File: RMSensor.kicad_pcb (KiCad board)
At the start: 2 copper layers, 32 x 32 mm, 26 parts, among them J1 Conn_01x02, J2 Conn_01x02, J3 Conn_01x04, U1 OPA209AID, U2 OPA2350UA, U3 MC78L05_SO8, U4 TLE2425xD

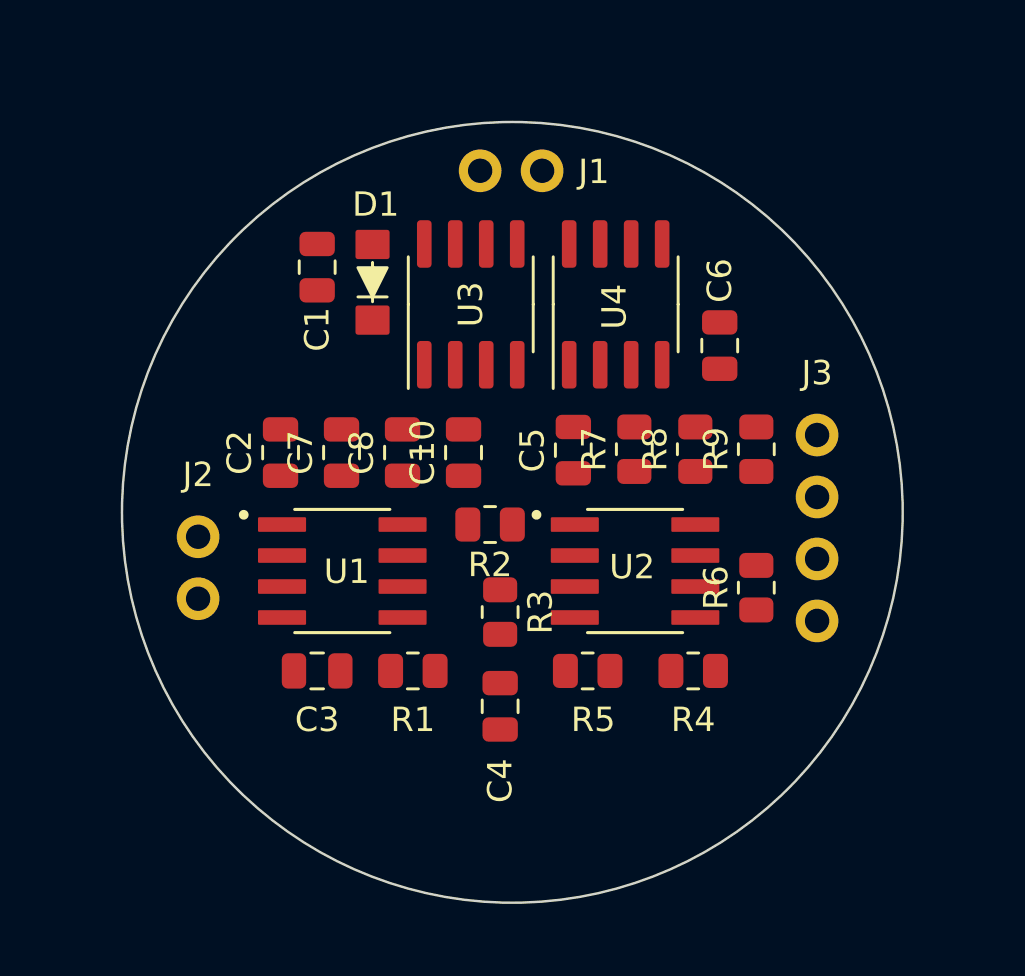
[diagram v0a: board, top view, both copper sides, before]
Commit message: pcb with traces
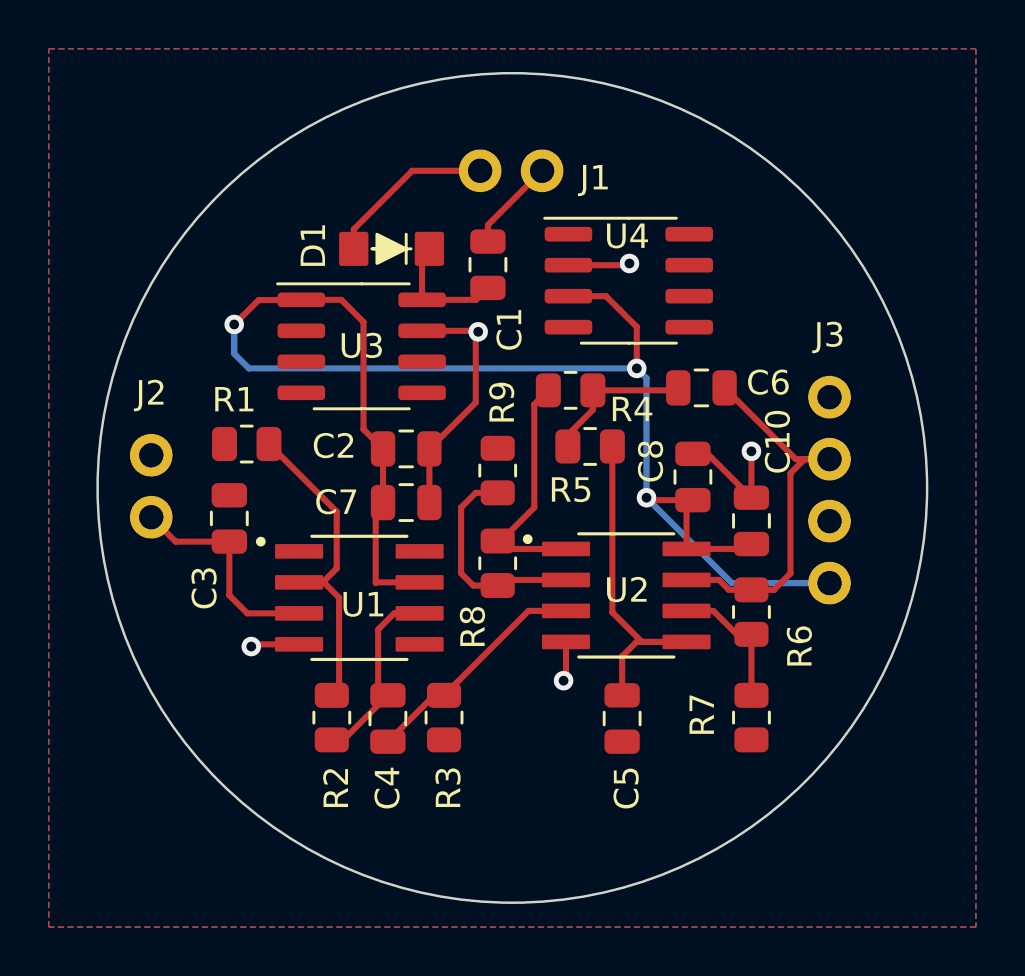
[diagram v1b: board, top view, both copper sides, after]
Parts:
- C2, C8: value 100n -> 1u
- moved R4 12.5 mm to (152.4, 96.0)
- moved C10 12.1 mm to (159.8, 101.3)
- moved R7 12.0 mm to (159.8, 109.4)
- moved C8 11.9 mm to (157.4, 99.5)
- moved R1 11.5 mm to (139.1, 98.2)
- moved C5 11.2 mm to (154.5, 109.5), turned to -90 degrees
- moved R9 10.6 mm to (149.4, 99.3), turned to -90 degrees
- moved R2 10.2 mm to (142.6, 109.4), turned to 90 degrees
- moved R8 9.35 mm to (149.4, 103.1)
- moved R5 9.20 mm to (153.2, 98.3)
- moved C3 7.21 mm to (138.4, 101.2), turned to 90 degrees
- moved C1 7.00 mm to (149.0, 90.8)
- moved C2 5.15 mm to (145.7, 98.4), turned to 0 degrees
- moved R3 4.90 mm to (147.2, 109.4)
- moved U3 4.79 mm to (143.8, 94.2), turned to 0 degrees
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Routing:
- net +5V: track 0.00 -> 63.4 mm, vias 0 -> 3
- net GND: track 0.00 -> 25.2 mm, vias 0 -> 5
- net Net-(C6-Pad2): track 0.00 -> 16.2 mm
- net Net-(C5-Pad1): track 0.00 -> 14.8 mm
- net Net-(R1-Pad2): track 0.00 -> 14.1 mm
- net Net-(R4-Pad2): track 0.00 -> 10.0 mm
- net Net-(C4-Pad1): track 0.00 -> 9.52 mm
- net Net-(R8-Pad1): track 0.00 -> 9.05 mm
- net Net-(C3-Pad1): track 0.00 -> 8.98 mm
- net Net-(C4-Pad2): track 0.00 -> 7.90 mm
- net Net-(D1-Pad2): track 0.00 -> 6.97 mm
- net Net-(C6-Pad1): track 0.00 -> 6.27 mm
- net Net-(R6-Pad1): track 0.00 -> 5.56 mm
- net Net-(C1-Pad1): track 0.00 -> 5.12 mm
- added copper zone on F.Cu, net +2V5
- added copper zone on B.Cu, net GND
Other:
- board size 32 x 32 mm -> 34 x 34 mm

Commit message: 31mm board
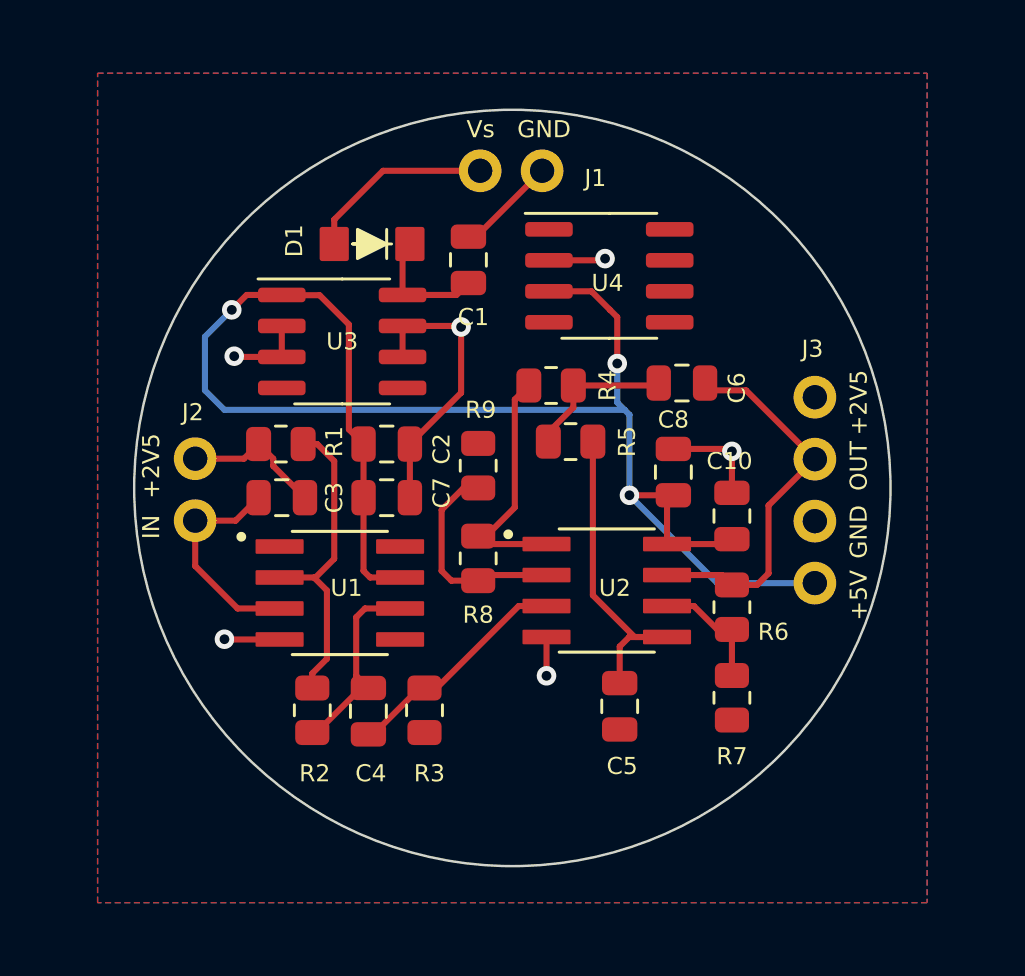
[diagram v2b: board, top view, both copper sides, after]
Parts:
- moved C3 2.31 mm to (140.6, 100.4), turned to 0 degrees
- moved J2 1.81 mm to (137.0, 100.1)
- moved R1 1.40 mm to (140.5, 98.2)
- moved R7 1.14 mm to (159.0, 108.6)
- moved C4 0.85 mm to (144.1, 109.2)
- moved R2 0.85 mm to (141.8, 109.1)
- moved R3 0.85 mm to (146.4, 109.1)
- moved C2 0.82 mm to (144.8, 98.2)
- moved C6 0.82 mm to (156.9, 95.7)
- moved C8 0.82 mm to (156.6, 99.3)
- moved D1 0.82 mm to (144.2, 90.0)
- moved R5 0.82 mm to (152.4, 98.1)
- moved R6 0.82 mm to (159.0, 104.9)
- moved R8 0.82 mm to (148.6, 102.9)
- moved C1 0.82 mm to (148.2, 90.7)
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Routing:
- net +2V5: track 0.39 -> 5.84 mm
- net GND: track 25.2 -> 29.3 mm, vias 5 -> 6
- net +5V: track 63.4 -> 65.3 mm
- net Net-(C5-Pad1): track 14.8 -> 13.6 mm
- net Net-(R1-Pad2): track 14.1 -> 13.1 mm
- net Net-(D1-Pad2): track 6.97 -> 7.81 mm
- net Net-(R6-Pad1): track 5.56 -> 4.95 mm
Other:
- board size 34 x 34 mm -> 31 x 31 mm
- board text added: "+2V5"
- board text added: "+5V"
- board text added: "GND"
- board text added: "IN"
- board text added: "OUT"
- board text added: "Vs"
